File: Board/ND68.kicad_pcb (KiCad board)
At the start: 2 copper layers, 68.6 x 41.9 mm, 38 parts, among them J1 USB_C_Receptacle_USB2.0_14P, J2 Conn_01x03_Pin, U1 NCP1117-3.3_SOT223, U2 RP2040, Y1 Crystal_GND24

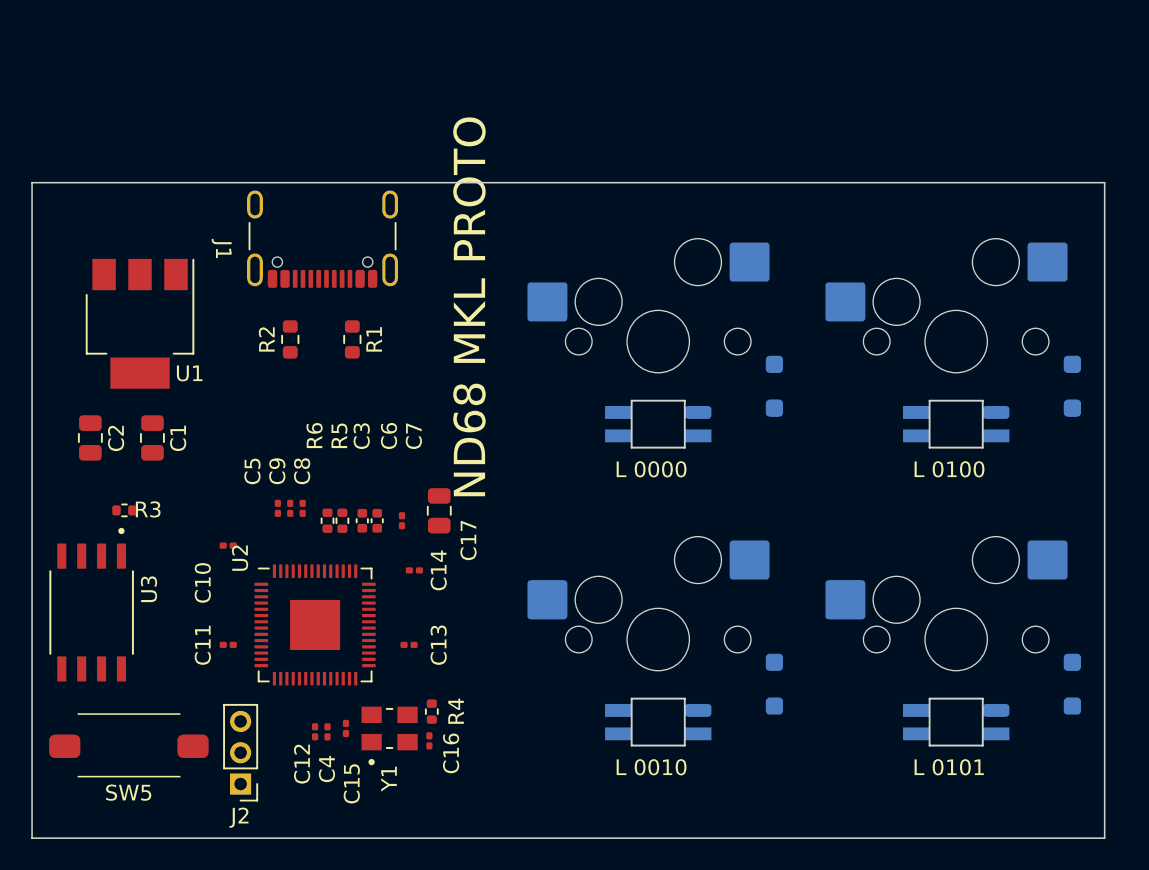
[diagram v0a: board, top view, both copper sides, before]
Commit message: Route mcu
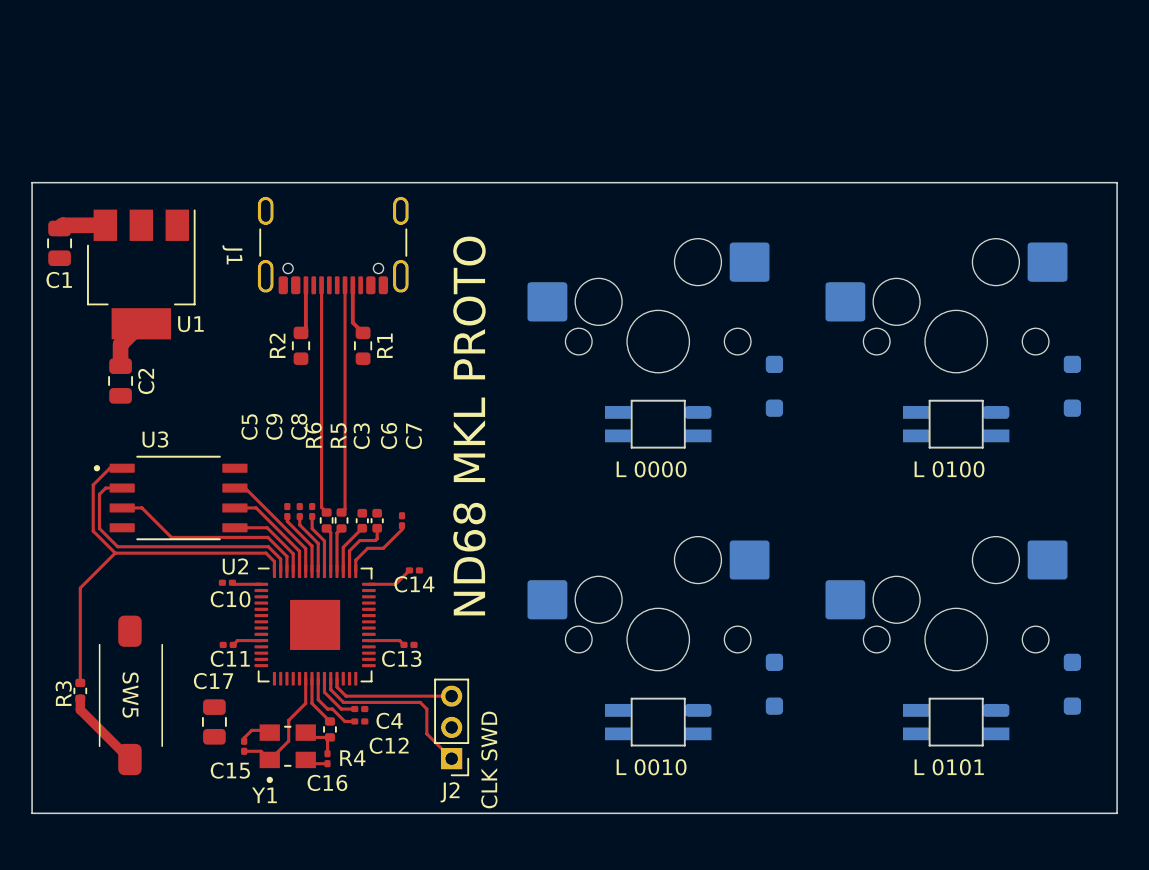
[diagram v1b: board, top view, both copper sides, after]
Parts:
- moved C17 19.7 mm to (141.2, 105.6), turned to -90 degrees
- moved C1 13.8 mm to (131.3, 75.0)
- moved J2 13.6 mm to (156.4, 108.0)
- moved R3 11.9 mm to (132.6, 103.6), turned to 90 degrees
- moved U3 9.19 mm to (138.9, 91.3), turned to 0 degrees
- moved C15 6.61 mm to (143.1, 107.2)
- moved C16 6.61 mm to (148.4, 108.0)
- moved R4 6.61 mm to (148.6, 106.1)
- moved Y1 6.61 mm to (145.9, 107.2)
- moved C2 4.12 mm to (135.2, 83.8)
- moved SW5 3.26 mm to (135.8, 103.9), turned to -90 degrees
- moved U1 3.15 mm to (136.5, 77.0)
- moved C12 2.93 mm to (150.5, 105.6), turned to 0 degrees
- moved C4 2.52 mm to (150.5, 104.8), turned to 0 degrees
- moved C10 2.38 mm to (142.0, 96.7)
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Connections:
- SW1 pad 5: (no net) -> Net-(D1-A)
- SW1 pad 6: (no net) -> C0
- SW2 pad 5: (no net) -> Net-(D2-A)
- SW2 pad 6: (no net) -> C1
- SW3 pad 5: (no net) -> Net-(D4-A)
- SW3 pad 6: (no net) -> C0
- SW4 pad 5: (no net) -> Net-(D3-A)
- SW4 pad 6: (no net) -> C1
- SW5 pad 1: (no net) -> GND
- SW5 pad 2: (no net) -> Net-(R3-Pad1)
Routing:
- net +3.3V: track 0.00 -> 33.3 mm
- net QSPI_SS: track 0.00 -> 27.5 mm
- net QSPI_SD1: track 0.00 -> 17.0 mm
- net D+: track 0.00 -> 14.7 mm
- net D-: track 0.00 -> 14.6 mm
- net QSPI_SD2: track 0.00 -> 12.8 mm
- net Net-(J2-Pin_1): track 0.00 -> 11.2 mm
- net +1V1: track 0.00 -> 10.6 mm
- net Net-(J2-Pin_3): track 0.00 -> 8.11 mm
- net XIN: track 0.00 -> 8.01 mm
- net QSPI_SD3: track 0.00 -> 7.57 mm
- net QSPI_SCLK: track 0.00 -> 6.55 mm
- net QSPI_SD0: track 0.00 -> 5.53 mm
- net Net-(R3-Pad1): track 0.00 -> 5.19 mm
- net GND: track 0.00 -> 3.60 mm
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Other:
- board size 68.6 x 41.9 mm -> 69.4 x 40.3 mm
- board text added: "CLK SWD"
